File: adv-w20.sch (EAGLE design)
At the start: 24 parts, among them Q1 NPN, Q2 NPN, U1 ESP32-WROOM, U2 L80-R, U3 CH340G, Y1 12MHz

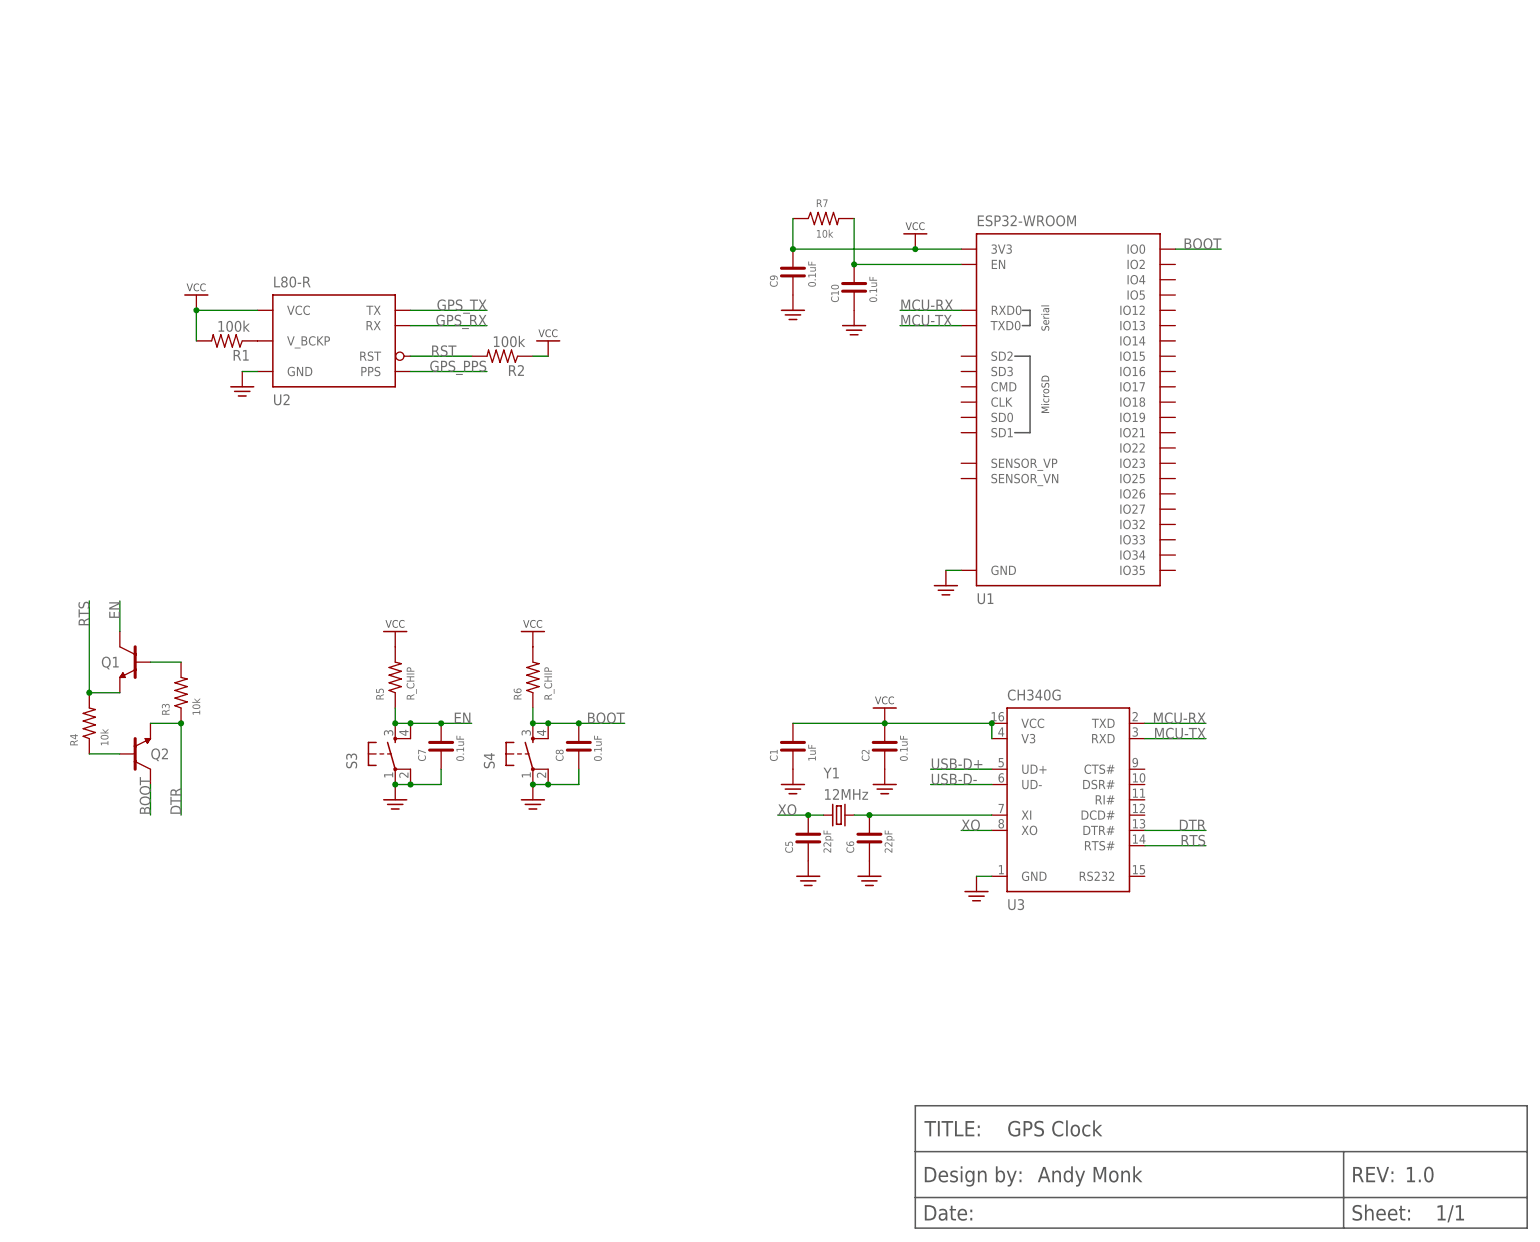
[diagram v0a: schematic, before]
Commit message: Add files via upload
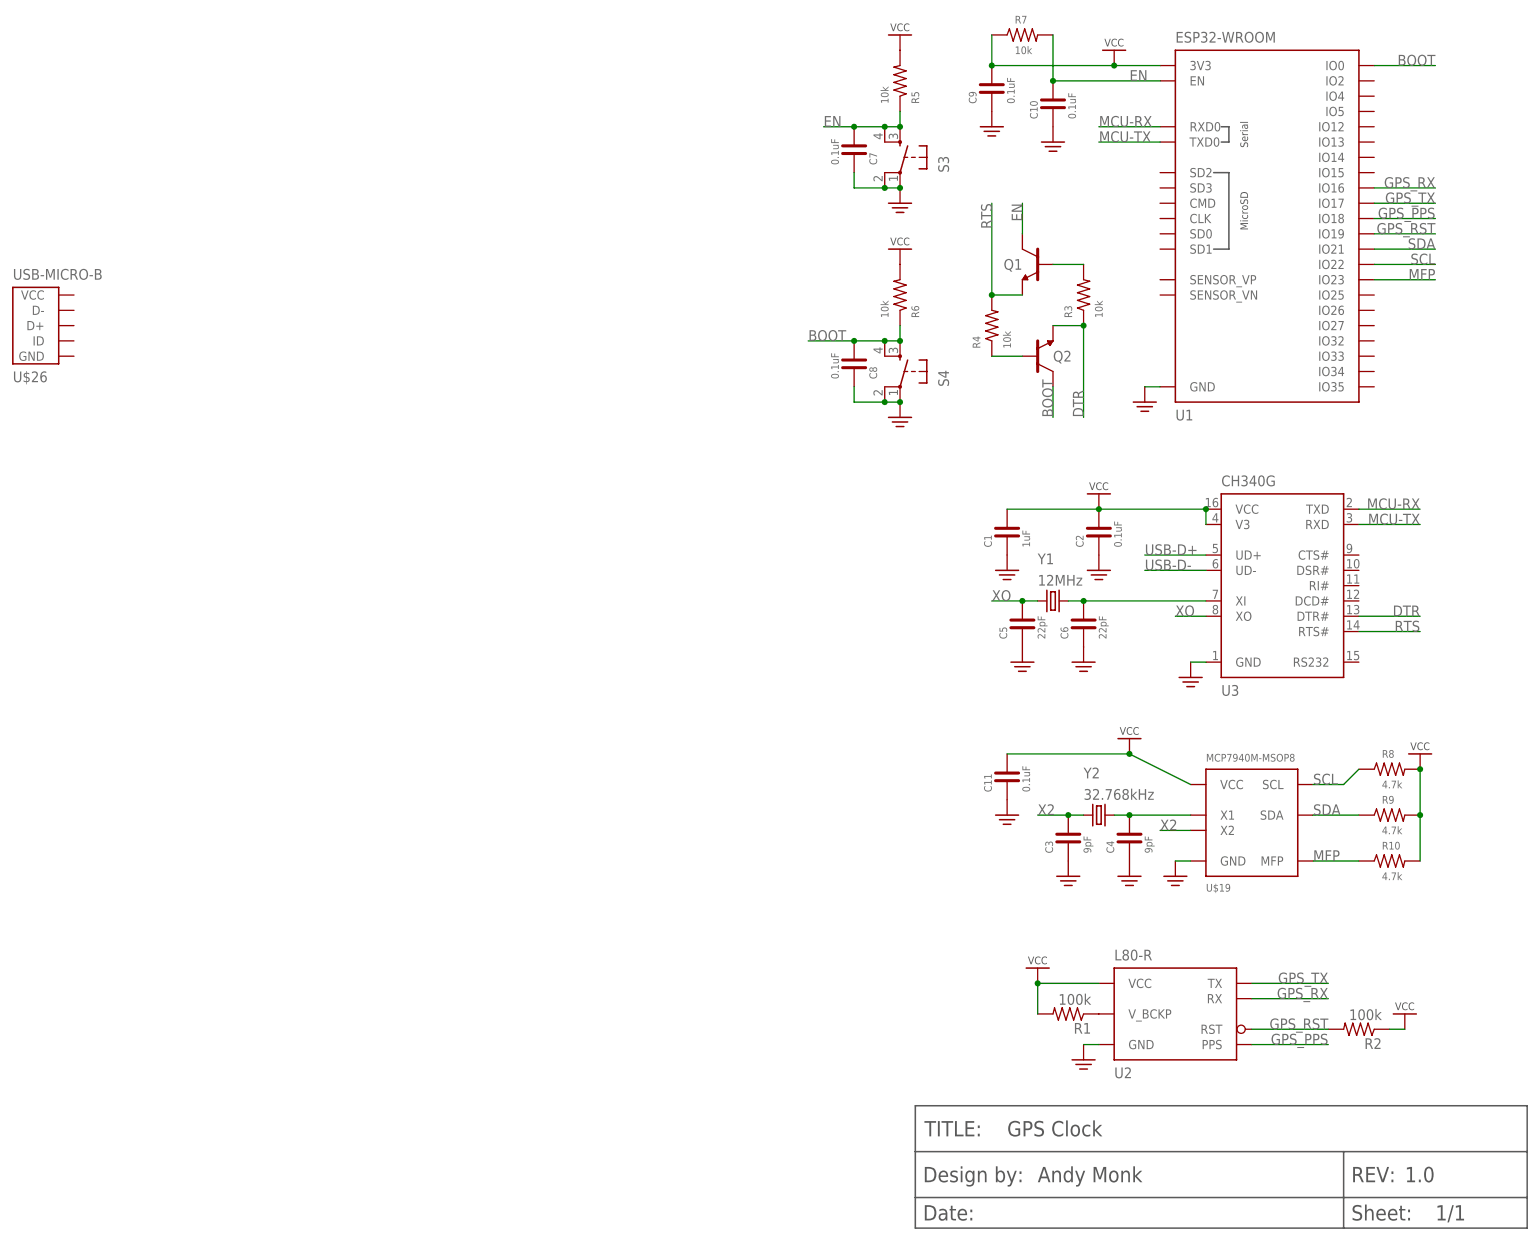
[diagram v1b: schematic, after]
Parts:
- added C11: 0.1uF, may2019-teaching:C_CHIP
- added C3, C4: 9pF, may2019-teaching:C_CHIP
- added R10, R8, R9: 4.7k, may2019-teaching:R_CHIP
- added U$19: MCP7940M-MSOP8, adv-w20:MCP7940M-MSOP8
- added U$26: USB-MICRO-B, may2019-teaching:USB-MICRO-B
- added Y2: 32.768kHz, adv-w20:XTAL
- R5, R6: value R_CHIP -> 10k
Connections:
- removed net N$6: C10.1, R7.2, U1.EN
- removed net RST: R2.2, U2.RST
- new net GPS_RST: R2.2, U1.IO19, U2.RST
- new net MFP: R10.1, U$19.MFP, U1.IO23
- new net N$3: C4.1, U$19.X1, Y2.2
- new net SCL: R8.1, U$19.SCL, U1.IO22
- new net SDA: R9.1, U$19.SDA, U1.IO21
- new net X2: C3.1, U$19.X2, Y2.1
- net EN: now also C10.1, R7.2, U1.EN
- net GND: now also C11.2, C3.2, C4.2, U$19.GND
- net GPS_PPS: now also U1.IO18
- net GPS_RX: now also U1.IO16
- net GPS_TX: now also U1.IO17
- net VCC: now also C11.1, R10.2, R8.2, R9.2, U$19.VCC
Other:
- moved on the sheet: C1, C10, C2, C5, C6, C7, C8, C9, Q1, Q2, R1, R2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
